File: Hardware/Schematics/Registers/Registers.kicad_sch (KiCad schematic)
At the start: 19 parts, among them J1 Conn_01x19, J2 Conn_01x08, J3 Conn_01x08, U1 74LS139, U10 74LS245, U11 74LS245, U12 74LS245, U13 74LS245, U14 74LS245, U15 74LS245, U16 74LS245, U2 74LS139, U3 74LS377, U4 74LS377, U5 74LS377, U6 74LS377, U7 74LS377, U8 74LS377, U9 74LS245

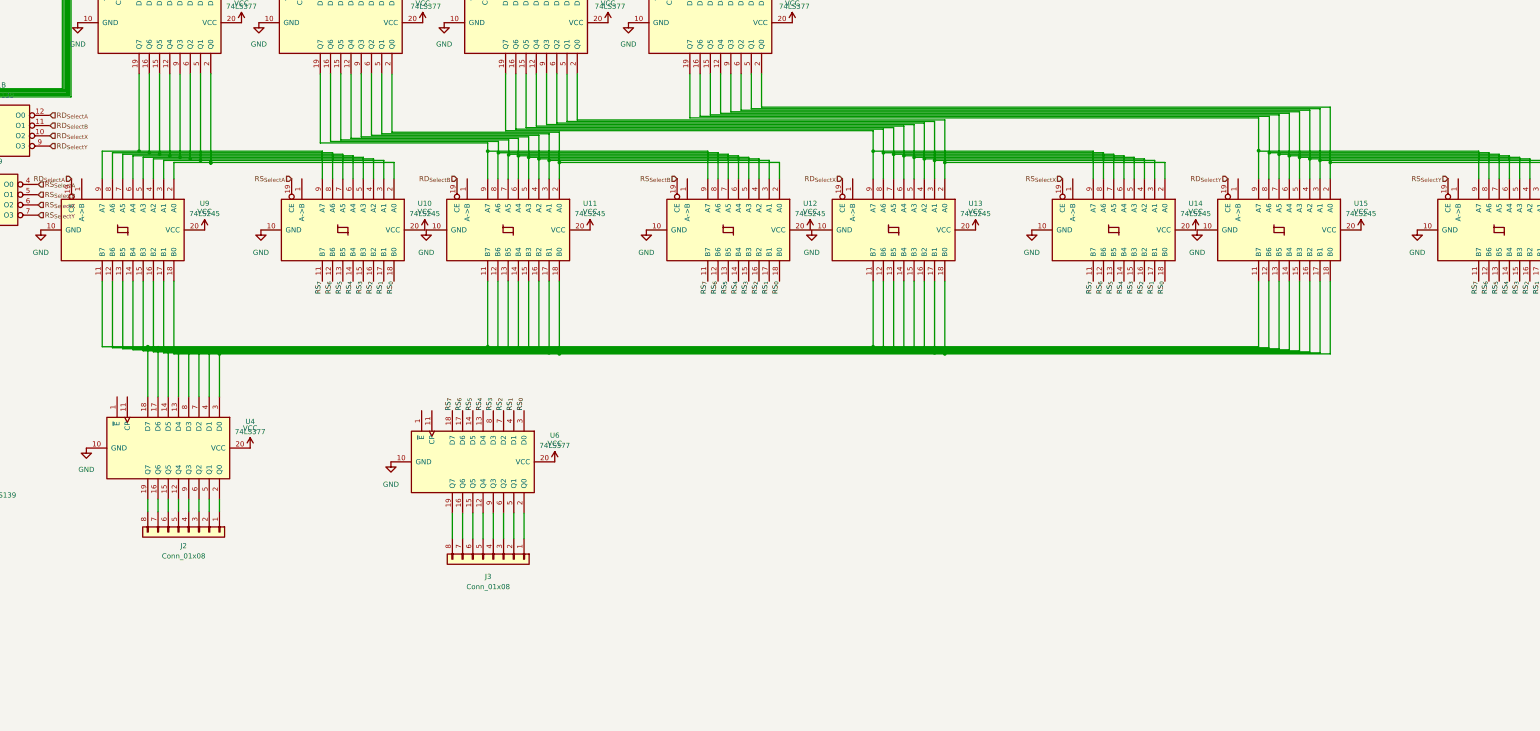
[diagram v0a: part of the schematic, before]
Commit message: Interim
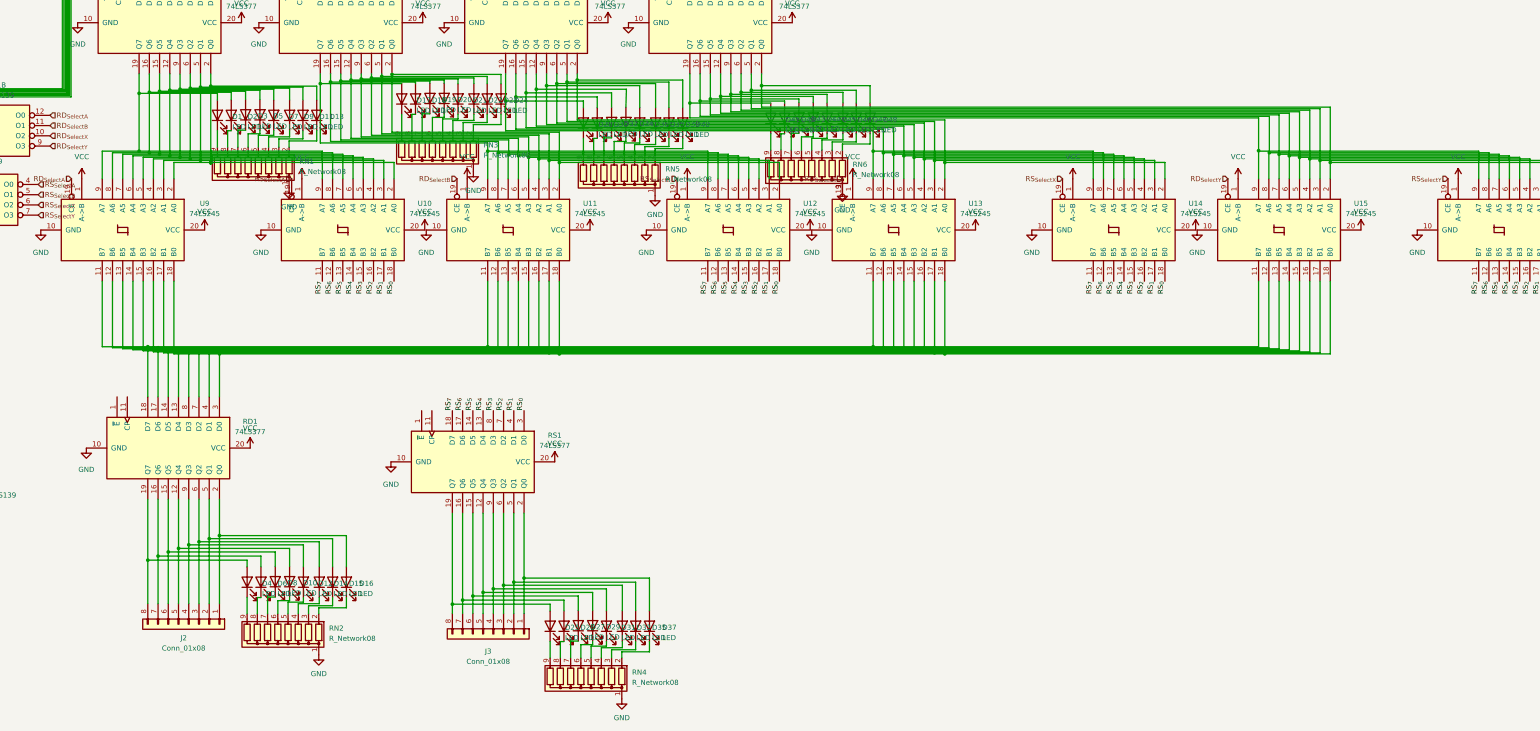
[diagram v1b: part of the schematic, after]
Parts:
- added D1, D10, D11, D12, D13, D14, D15, D16, D17, D18, D19, D2, D20, D21, D22, D23, D24, D25, D26, D27, D28, D29, D3, D30, D31, D32, D33, D34, D35, D36, D37, D38, D39, D4, D40, D41, D42, D43, D44, D45, D46, D47, D48, D5, D6, D7, D8, D9: LED, LED_THT:LED_D3.0mm, symbol Device:LED
- added RN1, RN2, RN3, RN4, RN5, RN6: R_Network08, Resistor_THT:R_Array_SIP9, symbol Device:R_Network08
- renumbered U4 to RD1, U6 to RS1
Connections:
- net GND: now also RN1.1 (common), RN2.1 (common), RN3.1 (common), RN4.1 (common), RN5.1 (common), RN6.1 (common)
- net VCC: now also U10.1 (A->B), U11.1 (A->B), U12.1 (A->B), U13.1 (A->B), U14.1 (A->B), U15.1 (A->B), U16.1 (A->B), U9.1 (A->B)
- net at U10.6 (A4), U3.12 (Q4), U9.6 (A4): now also D5.2 (A)
- net at U10.7 (A5), U3.15 (Q5), U9.7 (A5): now also D3.2 (A)
- net at U10.8 (A6), U3.16 (Q6), U9.8 (A6): now also D2.2 (A)
- net at U10.9 (A7), U3.19 (Q7), U9.9 (A7): now also D1.2 (A)
- net at U10.2 (A0), U3.2 (Q0), U9.2 (A0): now also D13.2 (A)
- net at U10.3 (A1), U3.5 (Q1), U9.3 (A1): now also D11.2 (A)
- net at U10.4 (A2), U3.6 (Q2), U9.4 (A2): now also D9.2 (A)
- net at U10.5 (A3), U3.9 (Q3), U9.5 (A3): now also D7.2 (A)
- net at U15.2 (A0), U16.2 (A0), U8.2 (Q0): now also D48.2 (A)
- net at U15.3 (A1), U16.3 (A1), U8.5 (Q1): now also D47.2 (A)
- net at U15.4 (A2), U16.4 (A2), U8.6 (Q2): now also D46.2 (A)
- net at U15.5 (A3), U16.5 (A3), U8.9 (Q3): now also D45.2 (A)
- net at U15.6 (A4), U16.6 (A4), U8.12 (Q4): now also D44.2 (A)
- net at U15.7 (A5), U16.7 (A5), U8.15 (Q5): now also D43.2 (A)
- net at U15.8 (A6), U16.8 (A6), U8.16 (Q6): now also D42.2 (A)
- net at U11.2 (A0), U12.2 (A0), U5.2 (Q0): now also D24.2 (A)
- net at U11.3 (A1), U12.3 (A1), U5.5 (Q1): now also D23.2 (A)
- net at U11.4 (A2), U12.4 (A2), U5.6 (Q2): now also D22.2 (A)
- net at U11.5 (A3), U12.5 (A3), U5.9 (Q3): now also D21.2 (A)
- net at U11.6 (A4), U12.6 (A4), U5.12 (Q4): now also D20.2 (A)
- net at U11.8 (A6), U12.8 (A6), U5.16 (Q6): now also D18.2 (A)
- net at U11.9 (A7), U12.9 (A7), U5.19 (Q7): now also D17.2 (A)
- net at J2.1 (Pin_1), RD1.2 (Q0): now also D16.2 (A)
- net at J2.2 (Pin_2), RD1.5 (Q1): now also D15.2 (A)
- net at J2.3 (Pin_3), RD1.6 (Q2): now also D14.2 (A)
- net at J2.4 (Pin_4), RD1.9 (Q3): now also D12.2 (A)
- net at J2.5 (Pin_5), RD1.12 (Q4): now also D10.2 (A)
- net at J2.6 (Pin_6), RD1.15 (Q5): now also D8.2 (A)
- net at J2.7 (Pin_7), RD1.16 (Q6): now also D6.2 (A)
- net at J2.8 (Pin_8), RD1.19 (Q7): now also D4.2 (A)
- net at U13.6 (A4), U14.6 (A4), U7.12 (Q4): now also D34.2 (A)
- net at U13.7 (A5), U14.7 (A5), U7.15 (Q5): now also D32.2 (A)
- net at U13.8 (A6), U14.8 (A6), U7.16 (Q6): now also D30.2 (A)
- net at U13.9 (A7), U14.9 (A7), U7.19 (Q7): now also D28.2 (A)
- net at U13.2 (A0), U14.2 (A0), U7.2 (Q0): now also D40.2 (A)
- net at U13.3 (A1), U14.3 (A1), U7.5 (Q1): now also D39.2 (A)
- net at U13.4 (A2), U14.4 (A2), U7.6 (Q2): now also D38.2 (A)
- net at U13.5 (A3), U14.5 (A3), U7.9 (Q3): now also D36.2 (A)
- net at J3.1 (Pin_1), RS1.2 (Q0): now also D37.2 (A)
- net at J3.2 (Pin_2), RS1.5 (Q1): now also D35.2 (A)
- net at J3.3 (Pin_3), RS1.6 (Q2): now also D33.2 (A)
- net at J3.4 (Pin_4), RS1.9 (Q3): now also D31.2 (A)
- net at J3.5 (Pin_5), RS1.12 (Q4): now also D29.2 (A)
- net at J3.6 (Pin_6), RS1.15 (Q5): now also D27.2 (A)
- net at J3.7 (Pin_7), RS1.16 (Q6): now also D26.2 (A)
- net at J3.8 (Pin_8), RS1.19 (Q7): now also D25.2 (A)
- net at U5.15 (Q5): now also D19.2 (A)
- net at U8.19 (Q7): now also D41.2 (A)
- new net: D47.1 (K), RN6.3 (R2)
- new net: D46.1 (K), RN6.4 (R3)
- new net: D45.1 (K), RN6.5 (R4)
- new net: D39.1 (K), RN5.3 (R2)
- new net: D5.1 (K), RN1.6 (R5)
- new net: D24.1 (K), RN3.2 (R1)
- new net: D23.1 (K), RN3.3 (R2)
- new net: D22.1 (K), RN3.4 (R3)
- new net: D21.1 (K), RN3.5 (R4)
- new net: D20.1 (K), RN3.6 (R5)
- new net: D19.1 (K), RN3.7 (R6)
- new net: D18.1 (K), RN3.8 (R7)
- new net: D17.1 (K), RN3.9 (R8)
- new net: D1.1 (K), RN1.9 (R8)
- new net: D43.1 (K), RN6.7 (R6)
- new net: D32.1 (K), RN5.7 (R6)
- new net: D8.1 (K), RN2.7 (R6)
- new net: D48.1 (K), RN6.2 (R1)
- new net: D16.1 (K), RN2.2 (R1)
- new net: D15.1 (K), RN2.3 (R2)
- new net: D14.1 (K), RN2.4 (R3)
- new net: D12.1 (K), RN2.5 (R4)
- new net: D10.1 (K), RN2.6 (R5)
- new net: D6.1 (K), RN2.8 (R7)
- new net: D4.1 (K), RN2.9 (R8)
- new net: D28.1 (K), RN5.9 (R8)
- new net: D13.1 (K), RN1.2 (R1)
- new net: D29.1 (K), RN4.6 (R5)
- new net: D2.1 (K), RN1.8 (R7)
- new net: D7.1 (K), RN1.5 (R4)
- new net: D11.1 (K), RN1.3 (R2)
- new net: D9.1 (K), RN1.4 (R3)
- new net: D3.1 (K), RN1.7 (R6)
- new net: D25.1 (K), RN4.9 (R8)
- new net: D34.1 (K), RN5.6 (R5)
- new net: D37.1 (K), RN4.2 (R1)
- new net: D35.1 (K), RN4.3 (R2)
- new net: D33.1 (K), RN4.4 (R3)
- new net: D31.1 (K), RN4.5 (R4)
- new net: D27.1 (K), RN4.7 (R6)
- new net: D26.1 (K), RN4.8 (R7)
- new net: D41.1 (K), RN6.9 (R8)
- new net: D42.1 (K), RN6.8 (R7)
- new net: D40.1 (K), RN5.2 (R1)
- new net: D38.1 (K), RN5.4 (R3)
- new net: D36.1 (K), RN5.5 (R4)
- new net: D30.1 (K), RN5.8 (R7)
- new net: D44.1 (K), RN6.6 (R5)
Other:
- moved on the sheet: J2, J3
